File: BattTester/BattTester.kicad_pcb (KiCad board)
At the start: 2 copper layers, 99.7 x 63.5 mm, 32 parts, among them J1 Battery, J2 SD_Card, J3 PWR, J4 UPDI, Q1 IRLZ44N, Q2 IRF4905, U1 LTC1286CN8, U2 ATtiny1624-SS, U3 LD1086DT33, U4 LM358AN

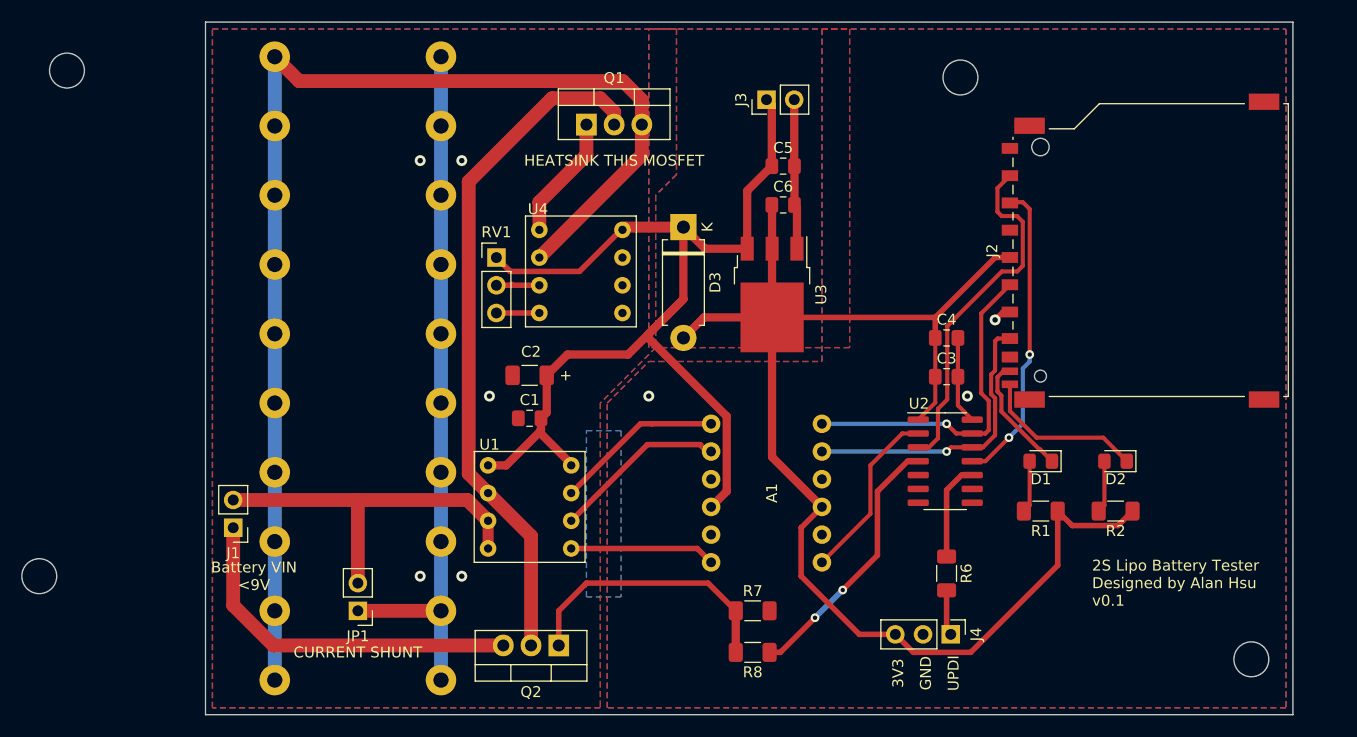
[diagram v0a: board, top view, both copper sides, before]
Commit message: work on things
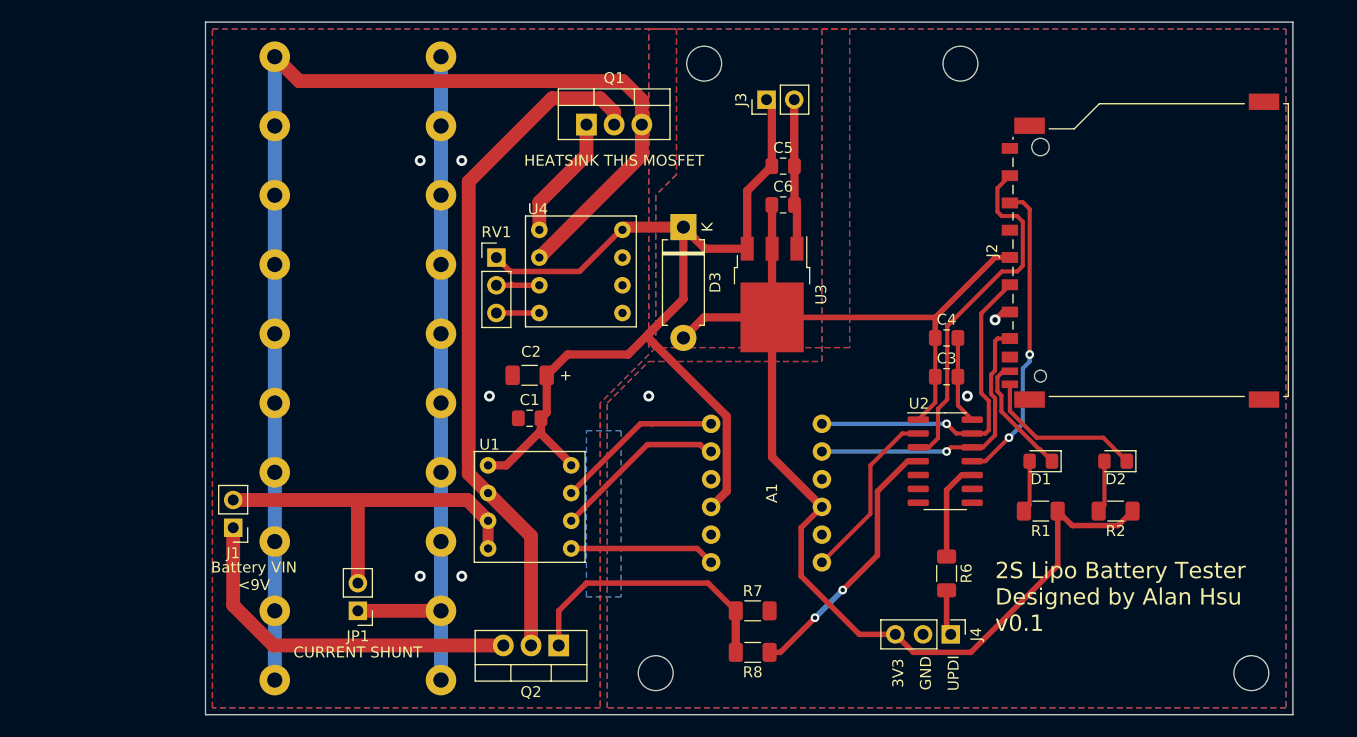
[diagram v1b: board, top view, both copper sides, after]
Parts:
- moved REF** 58.4 mm to (184.8, 67.3)
- moved REF** 57.2 mm to (180.3, 123.2)
- moved REF** 1.27 mm to (208.3, 67.3)
- moved REF** 1.27 mm to (234.9, 123.2)

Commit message: Fix #1
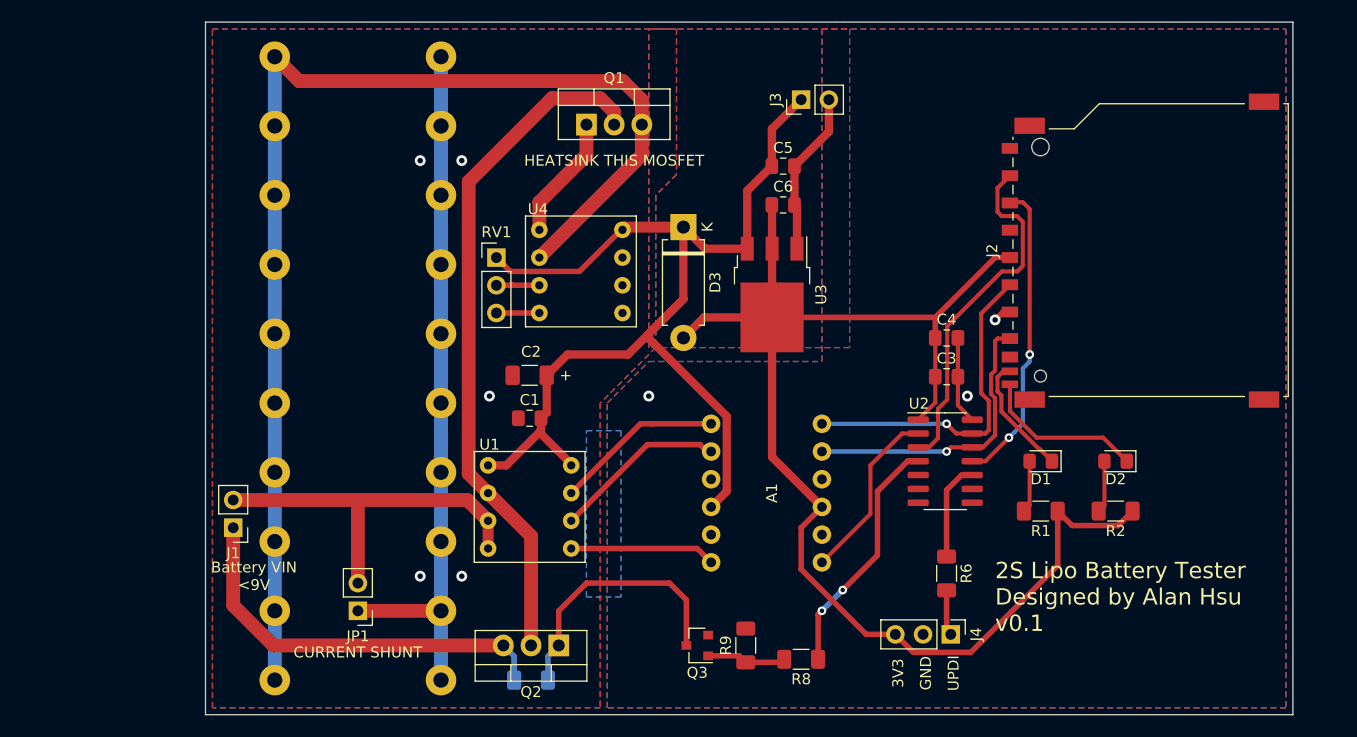
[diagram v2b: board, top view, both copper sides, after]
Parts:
- removed REF** (x4): MountingHole_3.2mm_M3, MountingHole:MountingHole_3.2mm_M3
- added Q3: 2N7002, Package_TO_SOT_SMD:SOT-23, F.Cu at (184.2, 120.7)
- added R9: 10K, Resistor_SMD:R_1206_3216Metric_Pad1.30x1.75mm_HandSolder, F.Cu at (188.6, 120.7)
- R7: moved to B.Cu
- moved R7 21.3 mm to (168.9, 123.8), turned to 180 degrees
- moved R8 4.49 mm to (193.7, 121.9)
- moved J3 3.18 mm to (193.7, 70.6)
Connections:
- R7 pad 2: GND -> /BIN+
- R8 pad 2: Net-(Q2-Pad1) -> Net-(Q3-Pad1)
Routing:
- net Net-(Q3-Pad1): track 0.00 -> 7.34 mm
- net /BIN+: track 33.4 -> 37.0 mm
- net /CUTOFF: track 24.3 -> 22.5 mm
- net GND: track 61.7 -> 63.0 mm
- net Net-(Q2-Pad1): track 25.3 -> 24.3 mm
- net +9V: track 103.0 -> 103.9 mm
